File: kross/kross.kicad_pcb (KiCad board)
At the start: 2 copper layers, 100 x 200 mm, 45 parts, among them J5 Synth_power_2x5

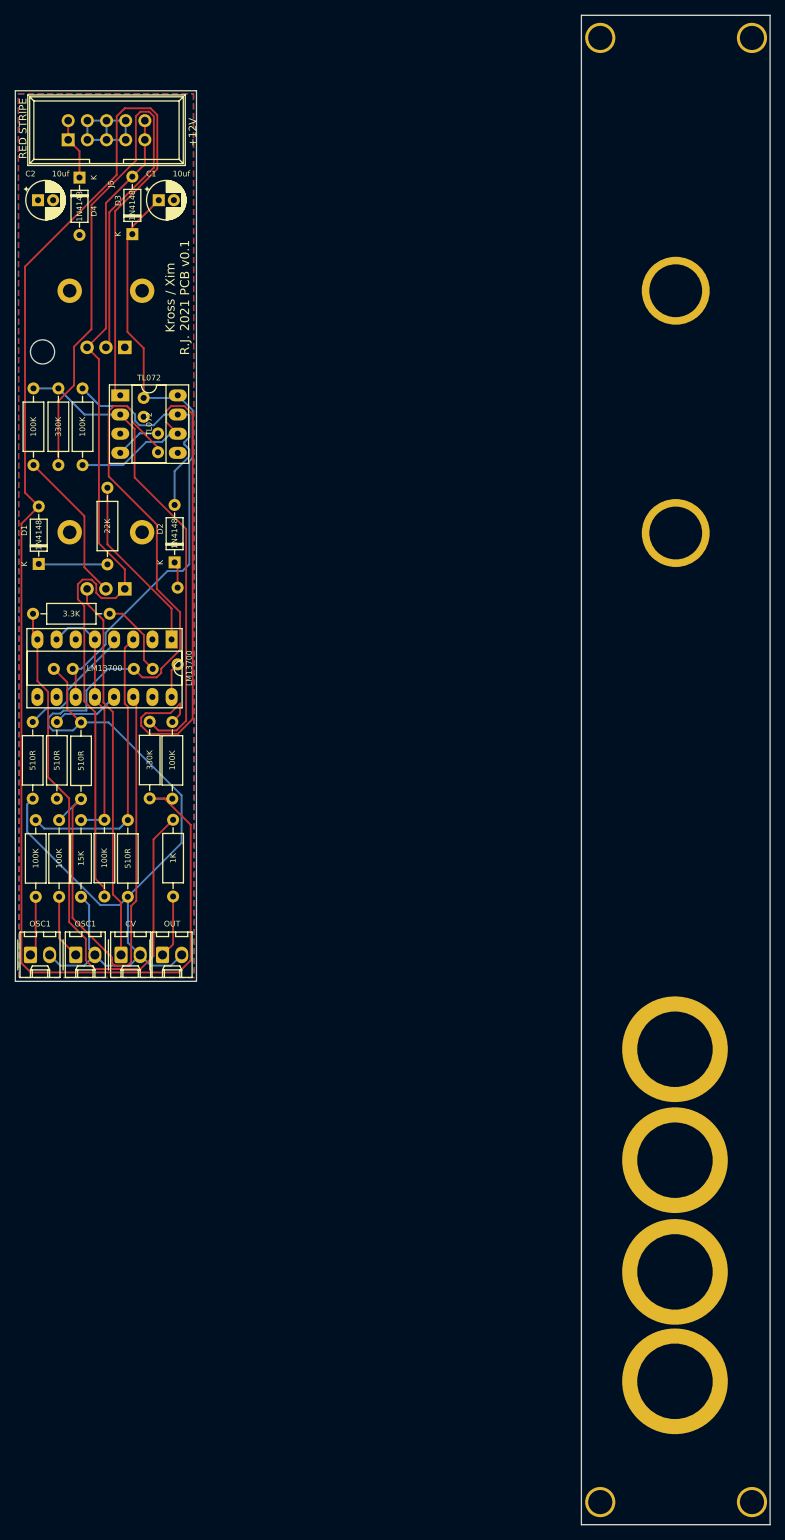
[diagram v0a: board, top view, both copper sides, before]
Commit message: sub work
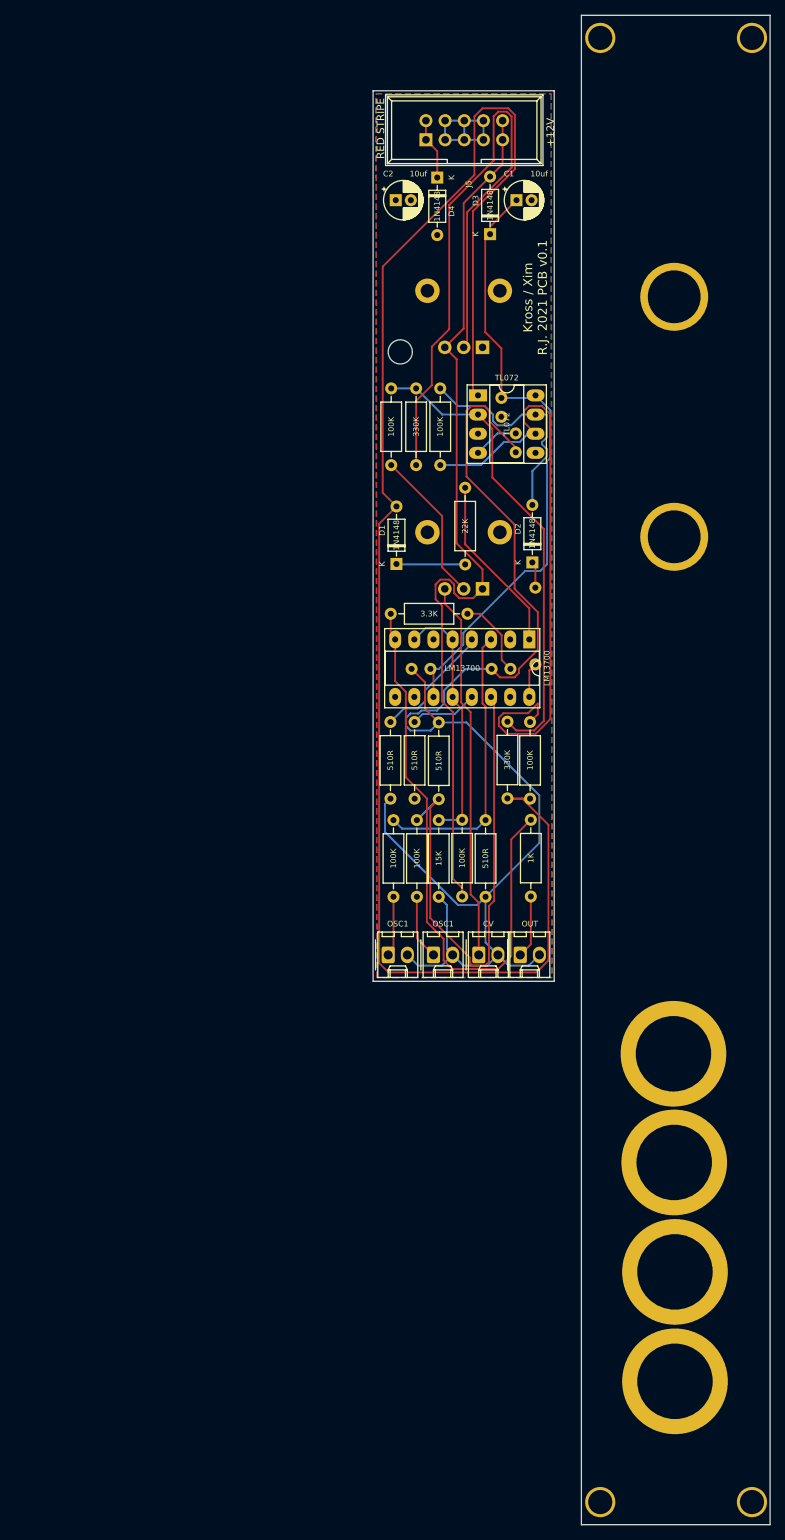
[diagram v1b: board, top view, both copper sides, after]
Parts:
- removed the REF** at (112.4, 157.0)
- removed the REF** at (112.4, 171.7)
- added REF**: Kosmo_Jack_Hole, ao_panel:Kosmo_Jack_Hole, F.Cu at (112.2, 157.6)
- added REF**: Kosmo_Jack_Hole, ao_panel:Kosmo_Jack_Hole, F.Cu at (112.3, 172.0)
- moved C1 47.4 mm to (91.4, 44.5)
- moved C2 47.4 mm to (75.4, 44.5)
- moved C3 47.4 mm to (89.4, 70.7)
- moved CV 47.4 mm to (86.4, 144.5)
- moved CVATTN1 47.4 mm to (84.4, 88.5)
- moved D3 47.4 mm to (87.9, 49.0)
- moved D4 47.4 mm to (80.9, 41.5)
- moved J5 47.4 mm to (79.4, 36.5)
- moved MIX1 47.4 mm to (84.4, 56.5)
- moved OSC1 47.4 mm to (74.4, 144.5)
- moved OSC1 47.4 mm to (80.4, 144.5)
- moved OUT 47.4 mm to (91.9, 144.5)
- moved R10 47.4 mm to (93.2, 123.8)
- moved R12 47.4 mm to (93.9, 106.0)
- moved R14 47.4 mm to (84.2, 126.6)
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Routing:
- net GND: track 196.6 -> 196.1 mm
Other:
- board size 100 x 200 mm -> 52.6 x 200 mm
